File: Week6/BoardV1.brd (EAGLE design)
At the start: 30.3 x 32.6 mm, 16 parts, among them IC1 ATTINY44-SSU

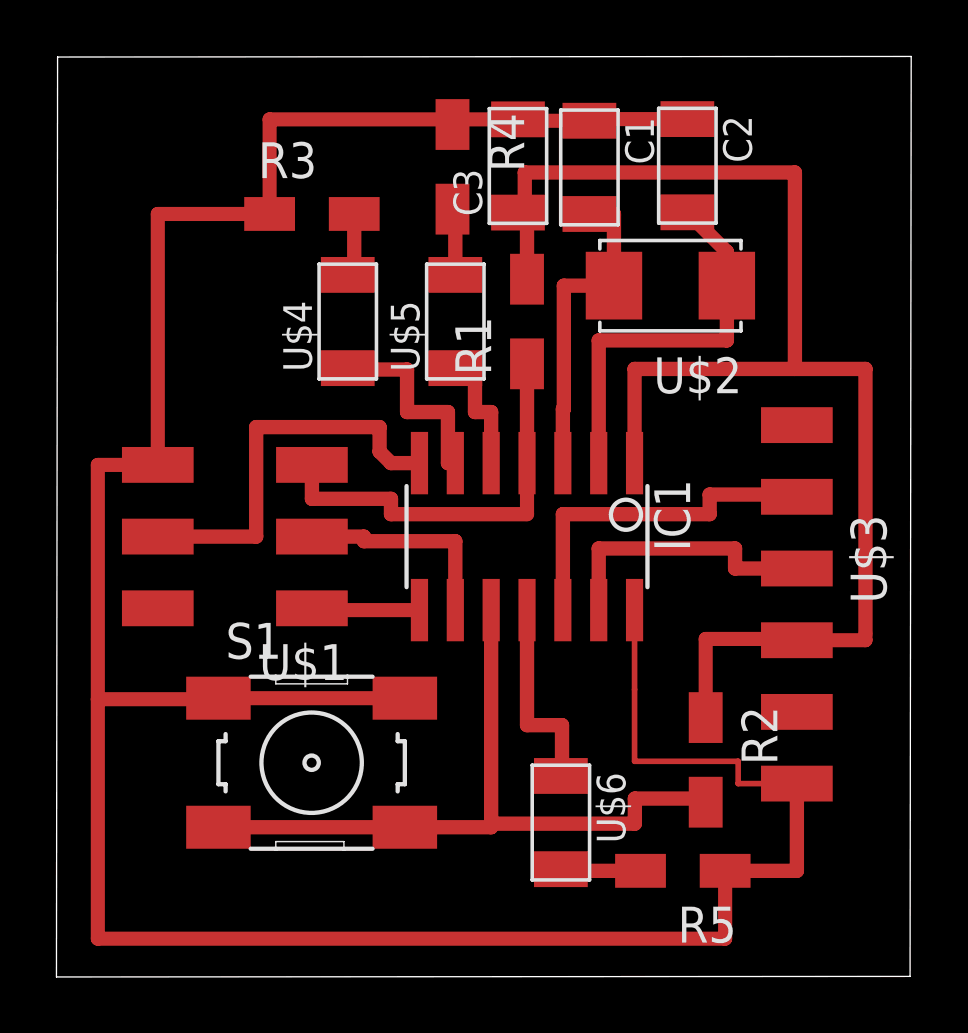
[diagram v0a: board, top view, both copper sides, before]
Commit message: la
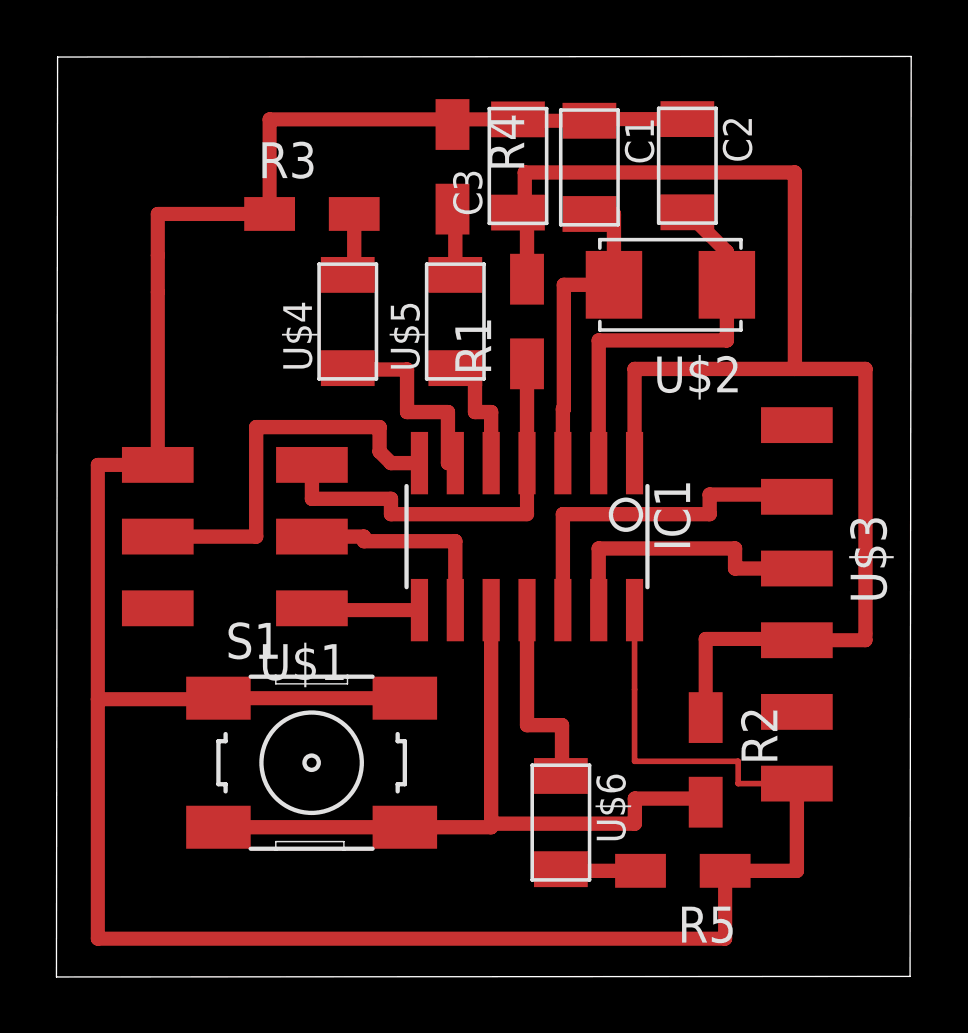
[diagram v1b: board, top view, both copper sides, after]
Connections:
- removed net N$7: U$1.2
- net VCC: now also U$1.2
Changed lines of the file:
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@@
 <layer number="17" name="Pads" color="2" fill="1" visible="yes" active="yes"/>
 <layer number="18" name="Vias" color="2" fill="1" visible="yes" active="yes"/>
-<layer number="19" name="Unrouted" color="6" fill="1" visible="yes" active="yes"/>
+<layer number="19" name="Unrouted" color="6" fill="1" visible="no" active="yes"/>
 <layer number="20" name="Dimension" color="24" fill="1" visible="yes" active="yes"/>
 <layer number="21" name="tPlace" color="7" fill="1" visible="yes" active="yes"/>
 <layer number="22" name="bPlace" color="7" fill="1" visible="yes" active="yes"/>
-<layer number="23" name="tOrigins" color="15" fill="1" visible="yes" active="yes"/>
+<layer number="23" name="tOrigins" color="15" fill="1" visible="no" active="yes"/>
 <layer number="24" name="bOrigins" color="15" fill="1" visible="yes" active="yes"/>
 <layer number="25" name="tNames" color="7" fill="1" visible="yes" active="yes"/>
 <layer number="26" name="bNames" color="7" fill="1" visible="yes" active="yes"/>
-<layer number="27" name="tValues" color="7" fill="1" visible="yes" active="yes"/>
+<layer number="27" name="tValues" color="7" fill="1" visible="no" active="yes"/>
 <layer number="28" name="bValues" color="7" fill="1" visible="yes" active="yes"/>
 <layer number="29" name="tStop" color="7" fill="3" visible="yes" active="yes"/>
@@
 <layer number="37" name="tTest" color="7" fill="1" visible="no" active="yes"/>
 <layer number="38" name="bTest" color="7" fill="1" visible="no" active="yes"/>
-<layer number="39" name="tKeepout" color="4" fill="11" visible="yes" active="yes"/>
+<layer number="39" name="tKeepout" color="4" fill="11" visible="no" active="yes"/>
 <layer number="40" name="bKeepout" color="1" fill="11" visible="yes" active="yes"/>
 <layer number="41" name="tRestrict" color="4" fill="10" visible="yes" active="yes"/>
@@
 <attribute name="VALUE" x="9.33" y="18.72" size="1.27" layer="27" rot="R180"/>
 </element>
-<element name="U$2" library="fabAca" package="2-SMD-5X3MM" value="CRYSTAL" x="20.76" y="22.53" smashed="yes" rot="R180">
-<attribute name="NAME" x="23.3" y="19.99" size="1.27" layer="25" rot="R180"/>
-<attribute name="VALUE" x="23.3" y="26.34" size="1.27" layer="27" rot="R180"/>
+<element name="U$2" library="fabAca" package="2-SMD-5X3MM" value="CRYSTAL" x="20.76" y="22.56" smashed="yes" rot="R180">
+<attribute name="NAME" x="23.3" y="20.02" size="1.27" layer="25" rot="R180"/>
+<attribute name="VALUE" x="23.3" y="26.37" size="1.27" layer="27" rot="R180"/>
 </element>
 <element name="U$3" library="fabAca" package="1X06SMD" value="FTDI-SMD-HEADER" x="25.24" y="11.24" smashed="yes" rot="R180">
@@
 <wire x1="6.561" y1="25.07" x2="6.561" y2="28.421" width="0.5" layer="1"/>
 <wire x1="6.561" y1="28.421" x2="13.04" y2="28.421" width="0.5" layer="1"/>
-<wire x1="2.6" y1="16.18" x2="2.6" y2="25.07" width="0.5" layer="1"/>
+<wire x1="2.6" y1="16.18" x2="2.6" y2="22.3" width="0.5" layer="1"/>
+<wire x1="2.6" y1="22.3" x2="2.6" y2="23.6" width="0.5" layer="1"/>
+<wire x1="2.6" y1="23.6" x2="2.6" y2="25.07" width="0.5" layer="1"/>
 <wire x1="2.6" y1="25.07" x2="6.561" y2="25.07" width="0.5" layer="1"/>
 <wire x1="2.6" y1="16.18" x2="0.476" y2="16.18" width="0.5" layer="1"/>
@@
 <wire x1="25.24" y1="10.015" x2="25.24" y2="9.97" width="0.5" layer="1"/>
 <wire x1="22.01" y1="7.229" x2="22.01" y2="10.015" width="0.5" layer="1"/>
+<contactref element="U$1" pad="2"/>
+<wire x1="2.6" y1="11.1" x2="15.68" y2="22.759" width="0" layer="19" extent="1-1"/>
 </signal>
 <signal name="RST">
@@
 <wire x1="16.95" y1="16.2435" x2="16.95" y2="18.157" width="0.508" layer="1"/>
 <wire x1="16.95" y1="18.157" x2="16.984" y2="18.157" width="0.508" layer="1"/>
-<wire x1="16.984" y1="22.53" x2="18.76" y2="22.53" width="0.508" layer="1"/>
-<wire x1="16.984" y1="18.157" x2="16.984" y2="22.53" width="0.508" layer="1"/>
-<wire x1="18.76" y1="22.53" x2="18.76" y2="25.069" width="0.508" layer="1"/>
+<wire x1="16.984" y1="22.56" x2="18.76" y2="22.56" width="0.508" layer="1"/>
+<wire x1="16.984" y1="18.157" x2="16.984" y2="22.56" width="0.508" layer="1"/>
+<wire x1="18.76" y1="22.56" x2="18.76" y2="25.069" width="0.508" layer="1"/>
 <wire x1="18.76" y1="25.069" x2="17.89" y2="25.069" width="0.508" layer="1"/>
 </signal>
@@
 <contactref element="IC1" pad="2"/>
 <contactref element="C2" pad="2"/>
-<wire x1="22.76" y1="22.53" x2="22.76" y2="23.729" width="0.508" layer="1"/>
+<wire x1="22.76" y1="22.56" x2="22.76" y2="23.729" width="0.508" layer="1"/>
 <wire x1="22.76" y1="23.729" x2="21.36" y2="25.129" width="0.508" layer="1"/>
-<wire x1="22.76" y1="20.59" x2="22.76" y2="22.53" width="0.508" layer="1"/>
+<wire x1="22.76" y1="20.59" x2="22.76" y2="22.56" width="0.508" layer="1"/>
 <wire x1="18.22" y1="16.2435" x2="18.22" y2="20.59" width="0.508" layer="1"/>
 <wire x1="18.22" y1="20.59" x2="22.76" y2="20.59" width="0.508" layer="1"/>
@@
 <wire x1="23.05" y1="13.22" x2="23.05" y2="12.51" width="0.508" layer="1"/>
 </signal>
-<signal name="N$7">
-<contactref element="U$1" pad="2"/>
-</signal>
 <signal name="LED2">
